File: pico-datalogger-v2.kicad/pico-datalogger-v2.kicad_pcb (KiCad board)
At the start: 2 copper layers, 46 x 60 mm, 35 parts, among them J1 JST-PH2 Bat, J10 Conn_PCB_2, J11 Conn_I2C1, J12 Conn_UART_5V, J13 Conn_I2C1, J14 Conn_I2C0, J2 Conn_Pico_Left, J3 Conn_Pico_Right, J4 Alt-Bat, J5 Conn_LoRa, J6 Conn_Display, J7 Conn_PCB_1, J8 Conn_ADC, J9 Conn_I2C0, Q1 AO3401A, Q2 AO3401A, SW1 SW_ON, SW2 SW_RUN, U1 74LVC2G74, U2 PCF8523T, U4 XTSD, Y1 Crystal

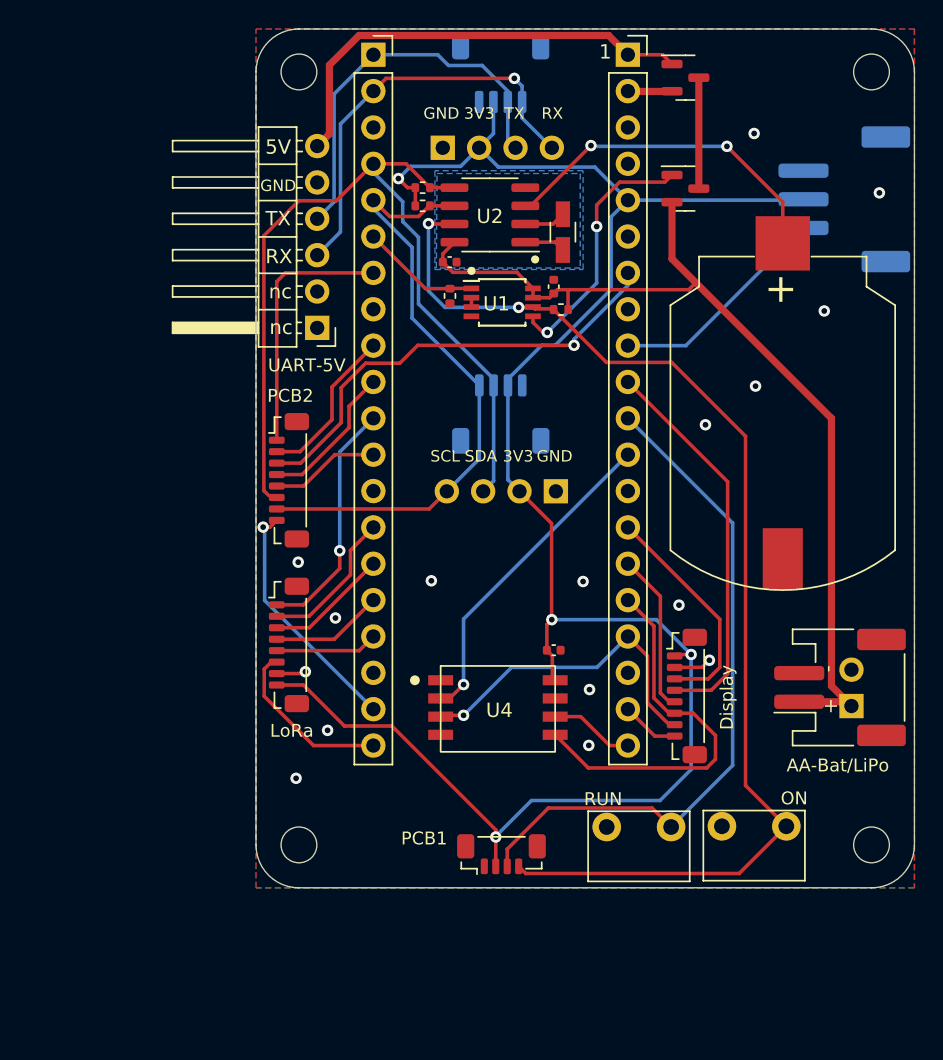
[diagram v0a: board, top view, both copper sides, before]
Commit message: added THT-connectors, finished routing
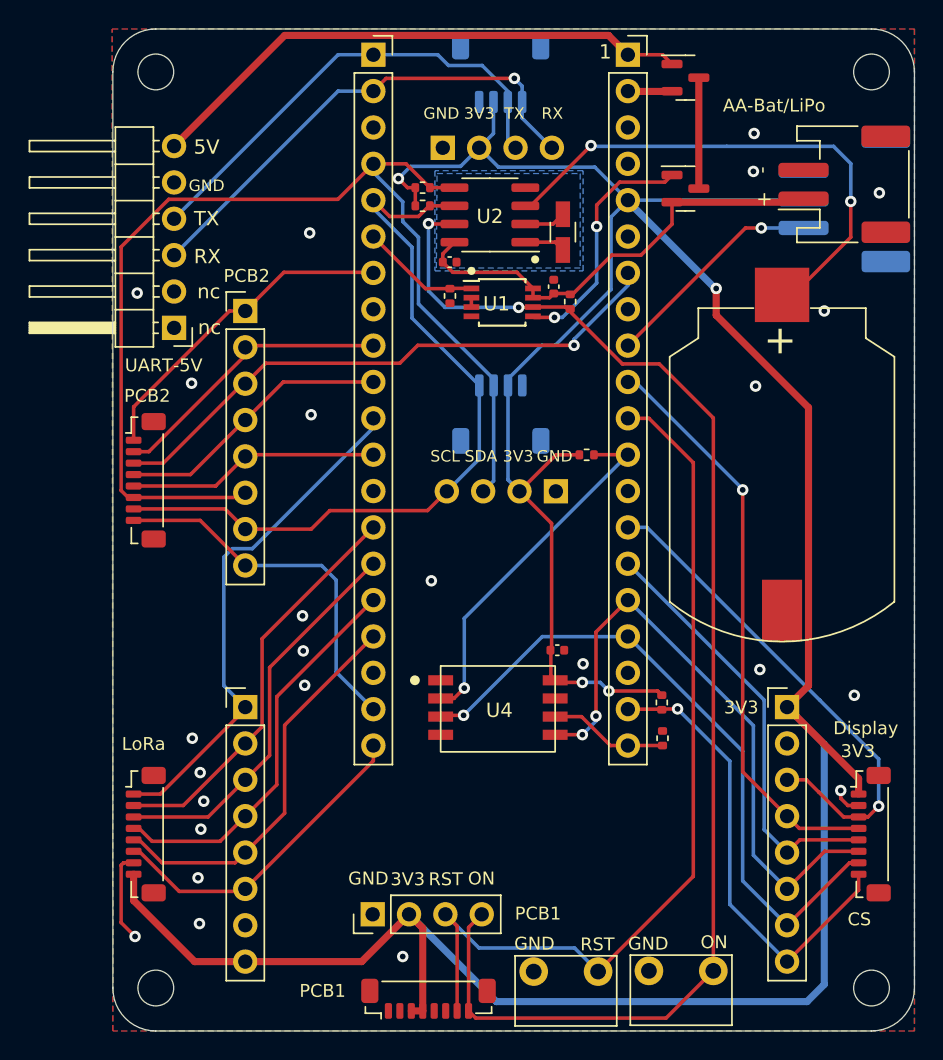
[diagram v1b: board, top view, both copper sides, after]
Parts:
- added J15: PCB_2_THT, Connector_PinHeader_2.54mm:PinHeader_1x08_P2.54mm_Vertical, F.Cu at (99.2, 119.7)
- added J16: LoRa_THT, Connector_PinHeader_2.54mm:PinHeader_1x08_P2.54mm_Vertical, F.Cu at (99.2, 147.4)
- added J17: Disp_THT, Connector_PinHeader_2.54mm:PinHeader_1x08_P2.54mm_Vertical, F.Cu at (137.1, 147.4)
- added R5: 10K, Resistor_SMD:R_0402_1005Metric, F.Cu at (128.3, 147.1)
- added R6: 100K, Resistor_SMD:R_0402_1005Metric, F.Cu at (128.4, 149.6)
- added R7: 10K, Resistor_SMD:R_0402_1005Metric, F.Cu at (123.1, 129.8)
- J4: value Alt-Bat -> PCB_1_THT; footprint Connector_PinHeader_2.54mm:PinHeader_1x02_P2.54mm_Vertical -> Connector_PinHeader_2.54mm:PinHeader_1x04_P2.54mm_Vertical; moved to F.Cu
- J7: footprint Connector_JST:JST_SUR_BM04B-SURS-TF_1x04-1MP_P0.80mm_Vertical -> Connector_JST:JST_SUR_BM08B-SURS-TF_1x08-1MP_P0.80mm_Vertical
- SW2: value SW_RUN -> SW_RST
- moved J4 36.5 mm to (108.2, 161.8), turned to 90 degrees
- moved J1 35.2 mm to (141.1, 110.8)
- moved J5 16.6 mm to (92.3, 156.2)
- moved J6 16.1 mm to (142.9, 156.2)
- moved H3 14.1 mm to (93.0, 167.0)
- moved SW1 11.3 mm to (127.5, 165.8)
- moved J7 11.3 mm to (112.0, 167.8)
- moved SW2 11.3 mm to (119.4, 165.8)
- moved H1 10.0 mm to (93.0, 103.0)
- moved H4 10.0 mm to (143.0, 167.0)
- moved J10 10.0 mm to (92.3, 131.5)
- moved J12 10.0 mm to (94.3, 120.9)
- moved BT1 3.60 mm to (136.8, 129.6)
- moved R2 0.85 mm to (122.0, 119.0), turned to -90 degrees
- moved C3 0.25 mm to (121.0, 143.4)
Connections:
- J4 pad 1: +BATT -> GND
- J4 pad 2: GND -> +3V3
- J7 pad 2: +3V3 -> GND
- J7 pad 3: /RUN -> +3V3
- J7 pad 4: /~{ON} -> +3V3
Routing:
- net +3V3: track 134.1 -> 223.5 mm
- net +BATT: track 66.7 -> 32.1 mm
- net /Display_CS: track 4.05 -> 32.5 mm, vias 0 -> 1
- net /SCLK0: track 23.1 -> 47.0 mm
- net /Lora_CS: track 7.16 -> 27.6 mm
- net /Lora_RST: track 7.88 -> 27.7 mm
- net /MISO1: track 16.9 -> 36.3 mm, vias 1 -> 0
- net /Display_RST: track 15.9 -> 35.3 mm, vias 0 -> 1
- net /MOSI1: track 8.60 -> 27.7 mm
- net /Display_DC: track 11.2 -> 30.1 mm
- net /SCLK1: track 10.3 -> 28.4 mm
- net /SDA: track 61.0 -> 79.1 mm
- net /MOSI0: track 27.0 -> 43.5 mm, vias 0 -> 2
- net /RUN: track 47.8 -> 63.6 mm
- net /Display_BUSY: track 27.5 -> 40.6 mm, vias 0 -> 1
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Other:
- board size 46 x 60 mm -> 56 x 70 mm
- board text added: "CS"
- board text added: "RST"
- board text removed: "RUN"
